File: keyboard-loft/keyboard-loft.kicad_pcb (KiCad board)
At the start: 2 copper layers, 24.1 x 11.2 mm, 2 parts, among them J1 Conn_01x04

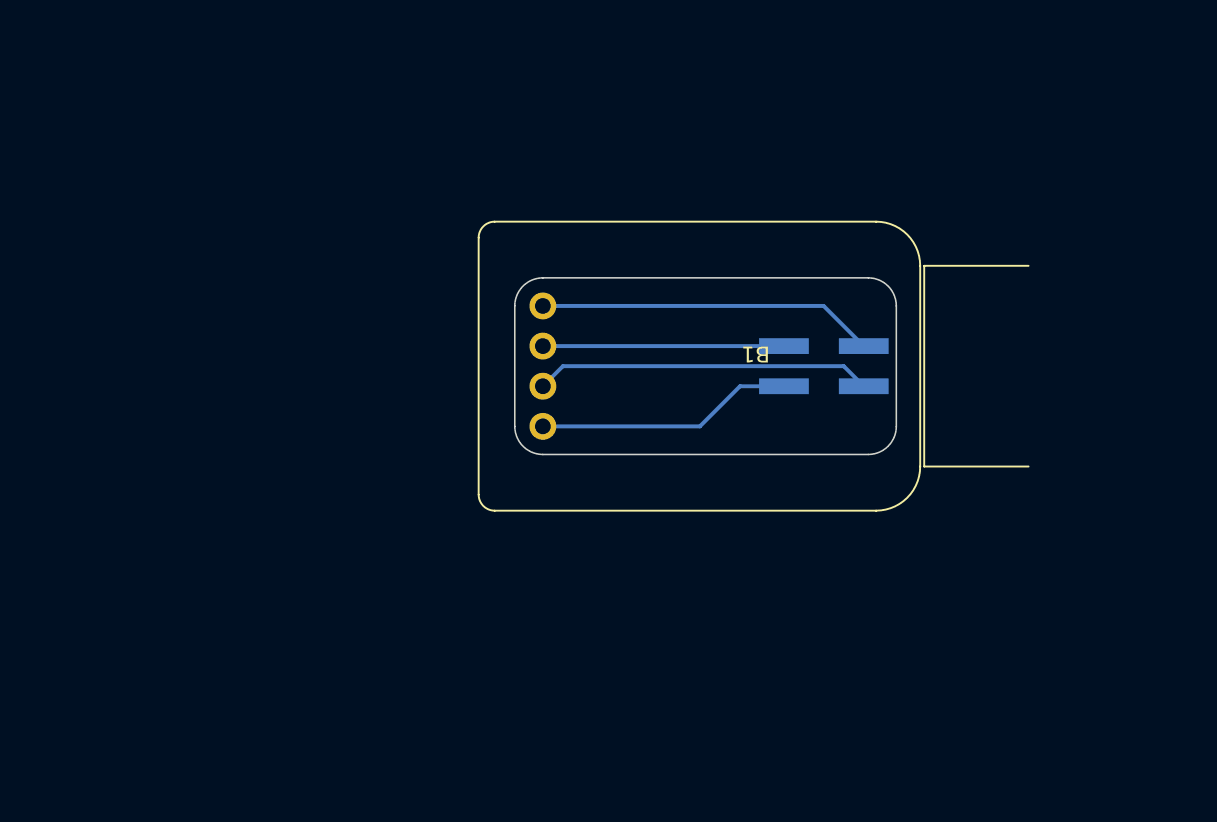
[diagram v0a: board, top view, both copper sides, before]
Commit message: current boards
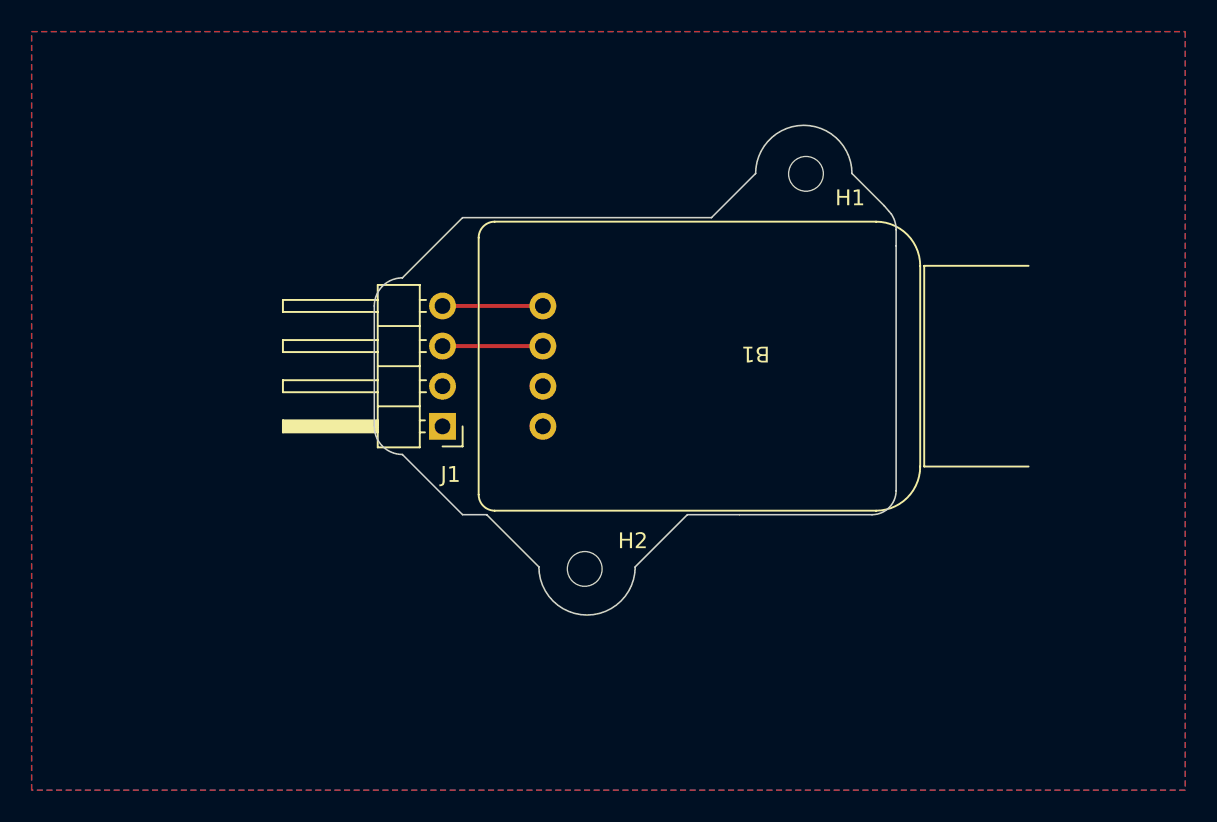
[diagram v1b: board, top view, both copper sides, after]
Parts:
- added H1: MountingHole, MountingHole:MountingHole_2.2mm_M2_ISO7380, F.Cu at (166.0, 78.0)
- added H2: MountingHole, MountingHole:MountingHole_2.2mm_M2_ISO7380, F.Cu at (152.0, 103.0)
- J1: footprint Connector_PinHeader_2.54mm:PinHeader_2x02_P2.54mm_Vertical_SMD -> Connector_PinHeader_2.54mm:PinHeader_1x04_P2.54mm_Horizontal; moved to F.Cu
- moved J1 24.4 mm to (143.0, 94.0), turned to 180 degrees
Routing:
- net /Vcc: track 21.4 -> 0.00 mm
- net /gnd: track 16.3 -> 0.00 mm
- net /Rx: track 21.4 -> 6.35 mm
- net /Tx: track 15.3 -> 6.35 mm
- added copper zone on F.Cu, net /Vcc
- added copper zone on B.Cu, net /gnd
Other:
- board size 24.1 x 11.2 mm -> 33 x 31 mm
